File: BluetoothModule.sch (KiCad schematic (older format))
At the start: 10 parts

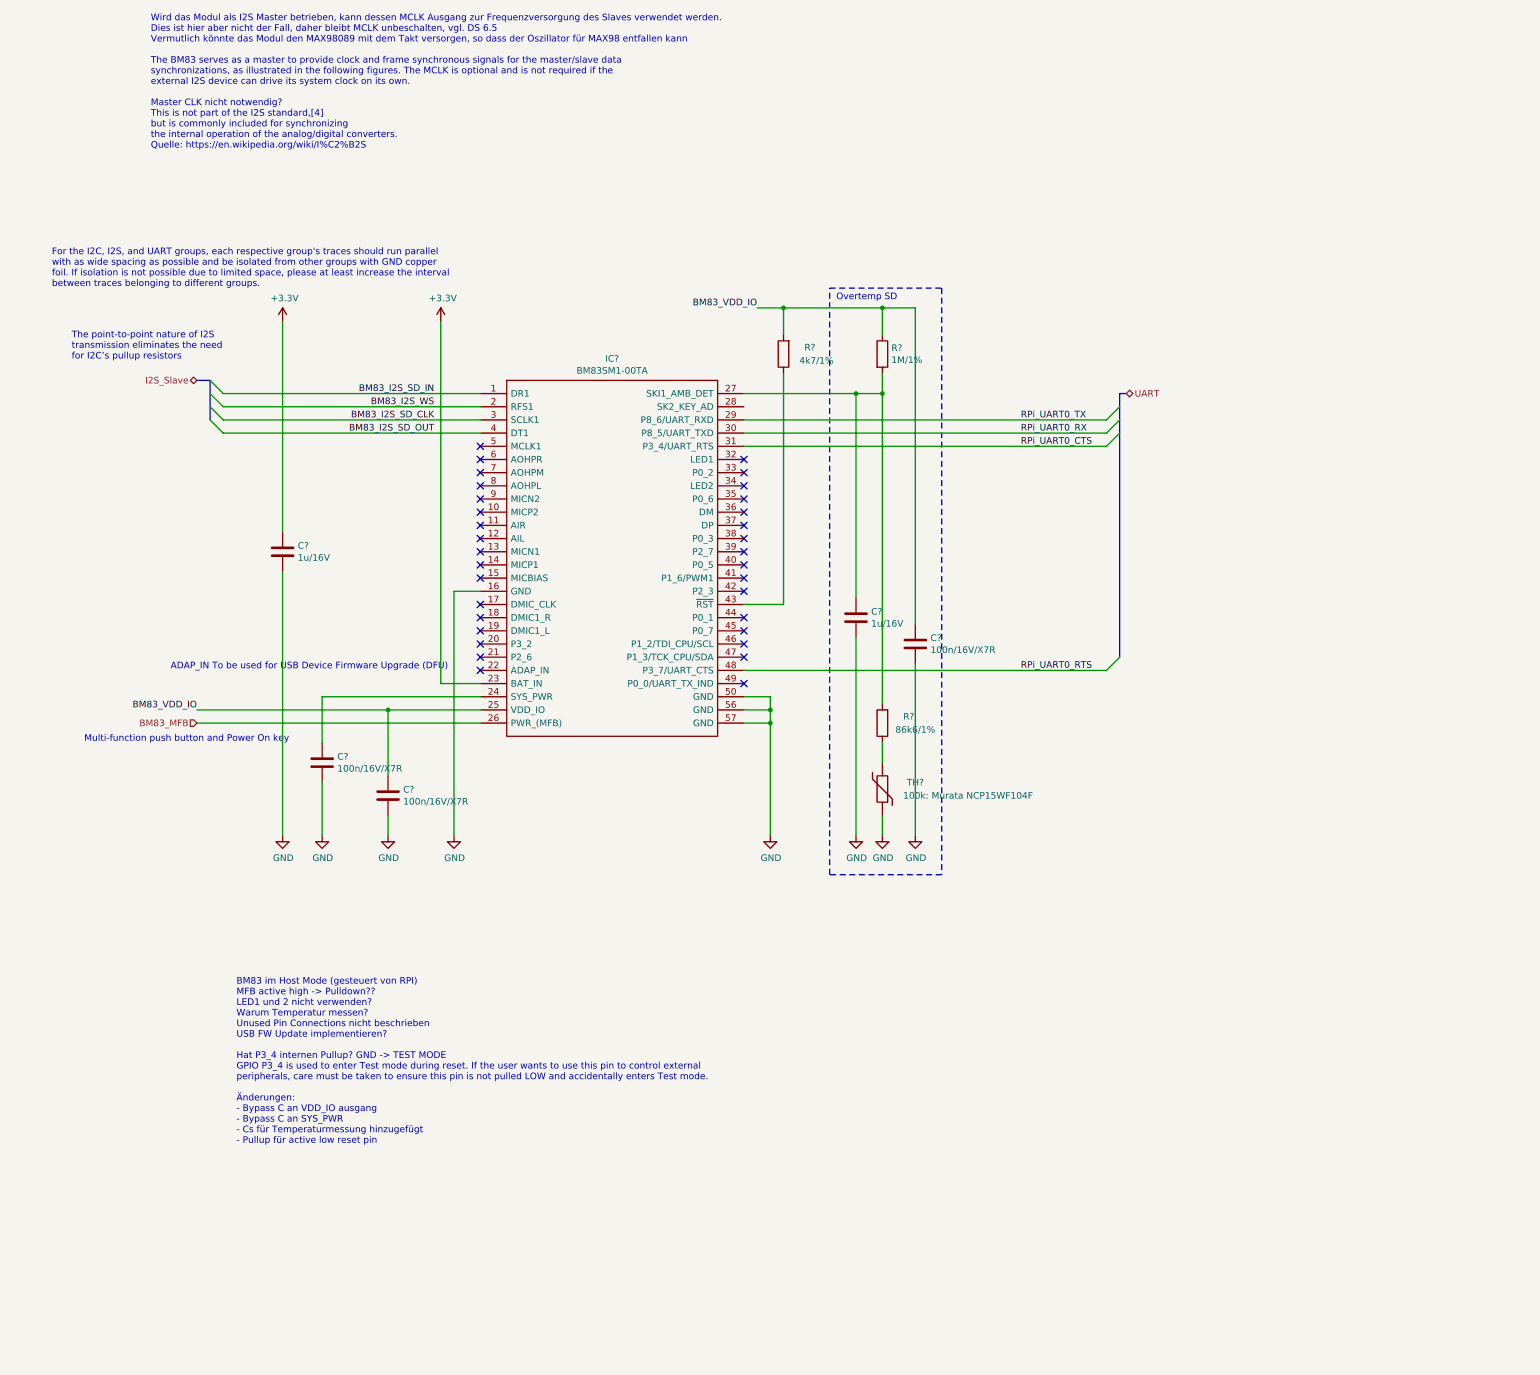
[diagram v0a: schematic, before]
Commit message: - BT fertig, warten auf Rueckmeldung von Microchip - CM3 fast fertig - diverse Kleinigkeiten
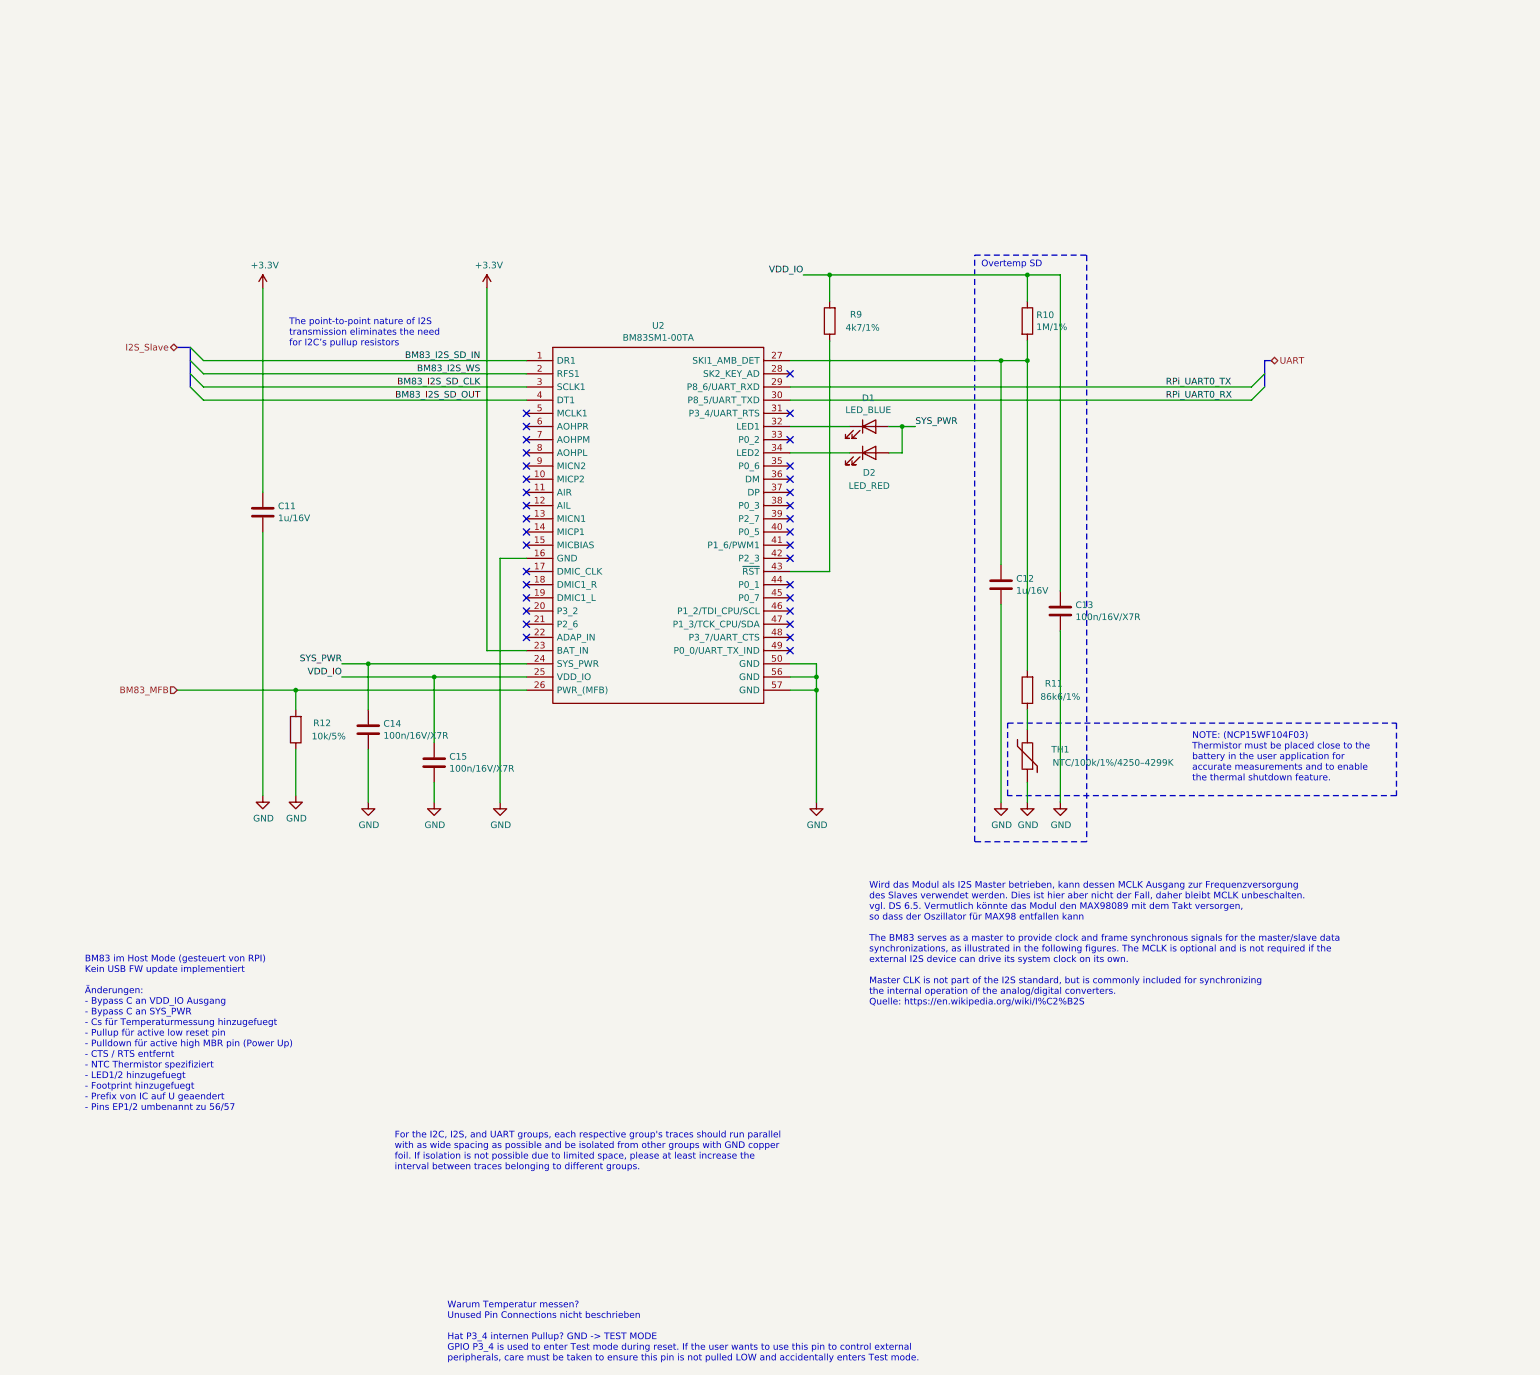
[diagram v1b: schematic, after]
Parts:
- added D1: LED_BLUE, LED_SMD:LED_0603_1608Metric, symbol Device:LED
- added D2: LED_RED, LED_SMD:LED_0603_1608Metric, symbol Device:LED
- added R12: 10k/5%, Resistor_SMD:R_0603_1608Metric, symbol Device:R
- R10, R11, R9: renamed from R?; footprint (none) -> Resistor_SMD:R_0603_1608Metric
- TH1: renamed from TH?; value 100k: Murata NCP15WF104F -> NTC/100k/1%/4250–4299K; footprint (none) -> Resistor_SMD:R_0603_1608Metric
- U2: renamed from IC?; footprint BM83SM100TA -> TeKaDe:BM83SM1
- gave numbers to parts that had none: 5
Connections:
- net BM83_MFB: now also R12.2
- net GND: now also R12.1
- net SYS_PWR: now reaches C14.1, U2.24 (SYS_PWR)
- net SYS_PWR: now also D1.2 (A), D2.2 (A)
- net at U2.32 (LED1): now also D1.1 (K)
- net at U2.34 (LED2): now also D2.1 (K)
- net BM83_VDD_IO renamed VDD_IO
- net RPi_UART0_CTS: no longer names the net of U2.31 (P3_4/UART_RTS)
- net RPi_UART0_RTS: no longer names the net of U2.48 (P3_7/UART_CTS)
- no-connect marks 33 -> 34
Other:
- note added: "BM83 im Host Mode (gesteuert von RPI)\nKein USB FW update implementiert\n\nÄnderungen:\n- Bypass C an VDD_IO Ausgang\n- Bypass C an SYS_PWR\n- Cs für Temperaturmessung hinzugefuegt\n- Pullup für active low reset pin\n- Pulldown für active high MBR pin (Power Up)\n- CTS / RTS entfernt\n- NTC Thermistor spezifiziert\n- LED1/2 hinzugefuegt\n- Footprint hinzugefuegt\n- Prefix von IC auf U geaendert\n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"
- note added: "For the I2C, I2S, and UART groups, each respective group's traces should run parallel\nwith as wide spacing as possible and be isolated from other groups with GND copper\nfoil. If isolation is not possible due to limited space, please at least increase the \ninterval between traces belonging to different groups."
- note added: "NOTE: (NCP15WF104F03)\nThermistor must be placed close to the\nbattery in the user application for\naccurate measurements and to enable\nthe thermal shutdown feature."
- note added: "Warum Temperatur messen?\nUnused Pin Connections nicht beschrieben\n\nHat P3_4 internen Pullup? GND -> TEST MODE\nGPIO P3_4 is used to enter Test mode during reset. If the user wants to use this pin to control external\nperipherals, care must be taken to ensure this pin is not pulled LOW and accidentally enters Test mode."
- note added: "Wird das Modul als I2S Master betrieben, kann dessen MCLK Ausgang zur Frequenzversorgung \ndes Slaves verwendet werden. Dies ist hier aber nicht der Fall, daher bleibt MCLK unbeschalten.\nvgl. DS 6.5. Vermutlich könnte das Modul den MAX98089 mit dem Takt versorgen, \nso dass der Oszillator für MAX98 entfallen kann\n\nThe BM83 serves as a master to provide clock and frame synchronous signals for t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"
- note removed: "ADAP_IN To be used for USB Device Firmware Upgrade (DFU)"
- note removed: "BM83 im Host Mode (gesteuert von RPI)\nMFB active high -> Pulldown??\nLED1 und 2 nicht verwenden?\nWarum Temperatur messen?\nUnused Pin Connections nicht beschrieben\nUSB FW Update implementieren?\n\nHat P3_4 internen Pullup? GND -> TEST MODE\nGPIO P3_4 is used to enter Test mode during reset. If the user wants to use this pin to control external\nperipherals, care must be taken to ensure this pi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"
- note removed: "For the I2C, I2S, and UART groups, each respective group's traces should run parallel\nwith as wide spacing as possible and be isolated from other groups with GND copper\nfoil. If isolation is not possible due to limited space, please at least increase the interval\nbetween traces belonging to different groups."
- note removed: "Multi-function push button and Power On key"
- note removed: "Wird das Modul als I2S Master betrieben, kann dessen MCLK Ausgang zur Frequenzversorgung des Slaves verwendet werden.\nDies ist hier aber nicht der Fall, daher bleibt MCLK unbeschalten, vgl. DS 6.5\nVermutlich könnte das Modul den MAX98089 mit dem Takt versorgen, so dass der Oszillator für MAX98 entfallen kann\n\nThe BM83 serves as a master to provide clock and frame synchronous signals for the m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"
- moved on the sheet: C11, C12, C13, C14, C15, R10, R11, R9, TH1, U2
